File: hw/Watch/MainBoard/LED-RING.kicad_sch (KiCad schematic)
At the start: 24 parts

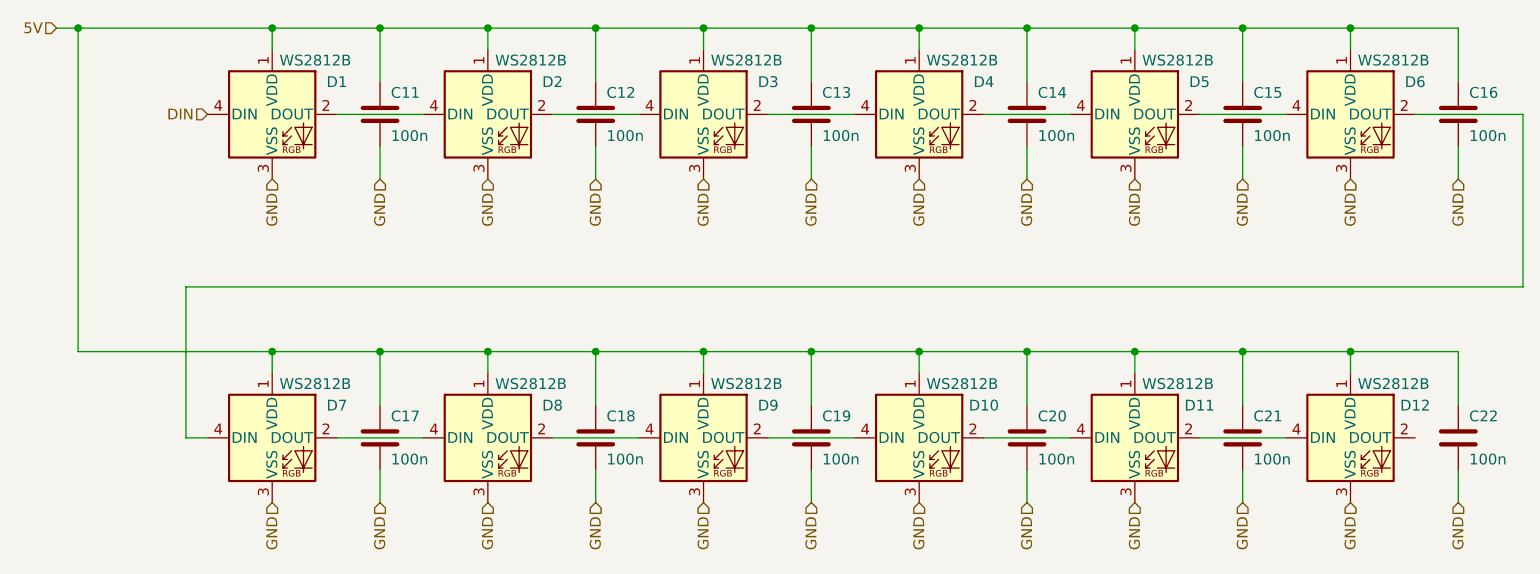
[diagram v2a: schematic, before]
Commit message: wip
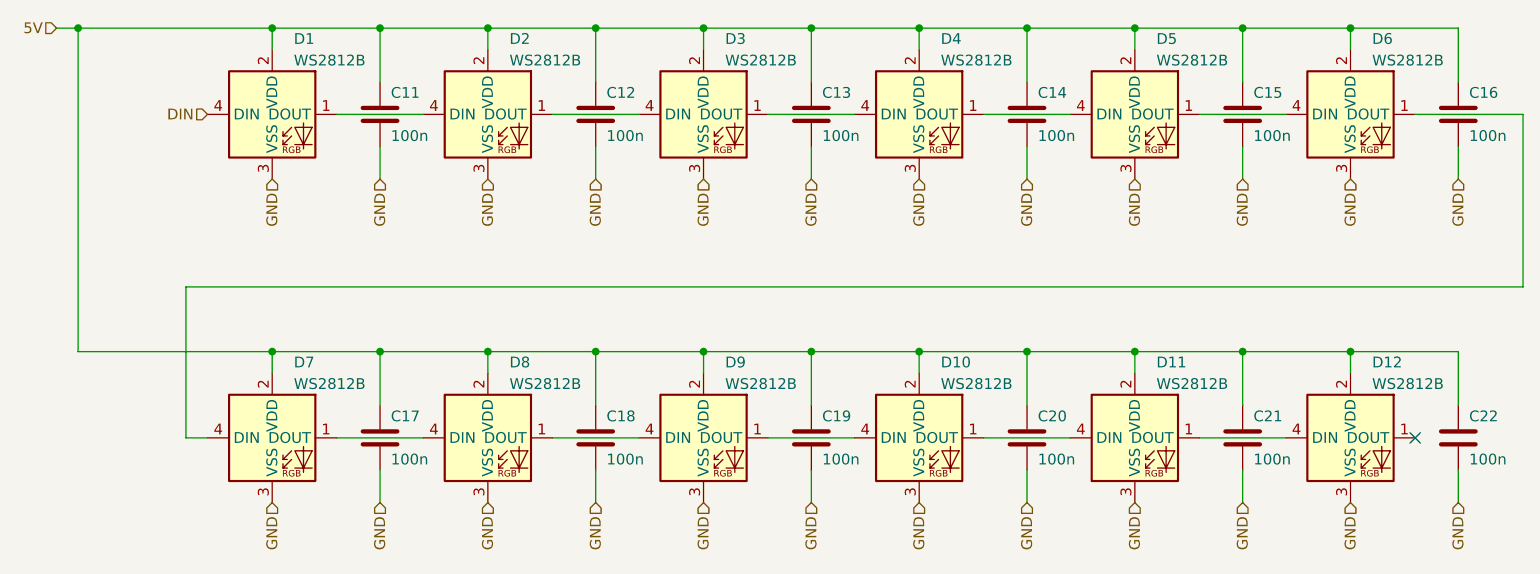
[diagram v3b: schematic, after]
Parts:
- removed D1, D10, D11, D12, D2, D3, D4, D5, D6, D7, D8, D9: WS2812B, RKL-LED:3528RGBW-WS2812B, symbol LED:WS2812B
- added D1, D10, D11, D12, D2, D3, D4, D5, D6, D7, D8, D9: WS2812B, RKL-LED:WS2812-1010, symbol RKL-Uncategorized:WS2812B
- C11, C12, C13, C14, C15, C16, C17, C18, C19, C20, C21, C22: footprint Capacitor_SMD:C_0402_1005Metric -> Capacitor_SMD:C_0201_0603Metric; Basic/Extended B -> E; LCSC C307331 -> C5142565; info 50V, X7R -> 10V, X5R
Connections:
- net 5V: now also D1.2 (VDD), D10.2 (VDD), D11.2 (VDD), D12.2 (VDD), D2.2 (VDD), D3.2 (VDD), D4.2 (VDD), D5.2 (VDD), D6.2 (VDD), D7.2 (VDD), D8.2 (VDD), D9.2 (VDD)
- net DIN: now also D1.4 (DIN)
- net GND: now also D1.3 (VSS), D10.3 (VSS), D11.3 (VSS), D12.3 (VSS), D2.3 (VSS), D3.3 (VSS), D4.3 (VSS), D5.3 (VSS), D6.3 (VSS), D7.3 (VSS), D8.3 (VSS), D9.3 (VSS)
- new net: D4.1 (DOUT), D5.4 (DIN)
- new net: D3.1 (DOUT), D4.4 (DIN)
- new net: D1.1 (DOUT), D2.4 (DIN)
- new net: D5.1 (DOUT), D6.4 (DIN)
- new net: D6.1 (DOUT), D7.4 (DIN)
- new net: D8.1 (DOUT), D9.4 (DIN)
- new net: D7.1 (DOUT), D8.4 (DIN)
- new net: D10.1 (DOUT), D11.4 (DIN)
- new net: D10.4 (DIN), D9.1 (DOUT)
- new net: D2.1 (DOUT), D3.4 (DIN)
- new net: D11.1 (DOUT), D12.4 (DIN)
- no-connect marks 0 -> 1

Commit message: PCB
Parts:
- C11, C12, C13, C14, C15, C16, C17, C18, C19, C20, C21, C22: footprint Capacitor_SMD:C_0201_0603Metric -> Capacitor_SMD:C_0402_1005Metric; Basic/Extended E -> B; LCSC C5142565 -> C307331; info 10V, X5R -> 50V, X7R
